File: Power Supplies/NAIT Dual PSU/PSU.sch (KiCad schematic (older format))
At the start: 41 parts, among them P1 120V, SW1 SW_Push_DPDT, SW2 SW_SPST_Lamp, T1 50V CT 100VA, U1 LM317_TO-220, U2 LM337_TO220

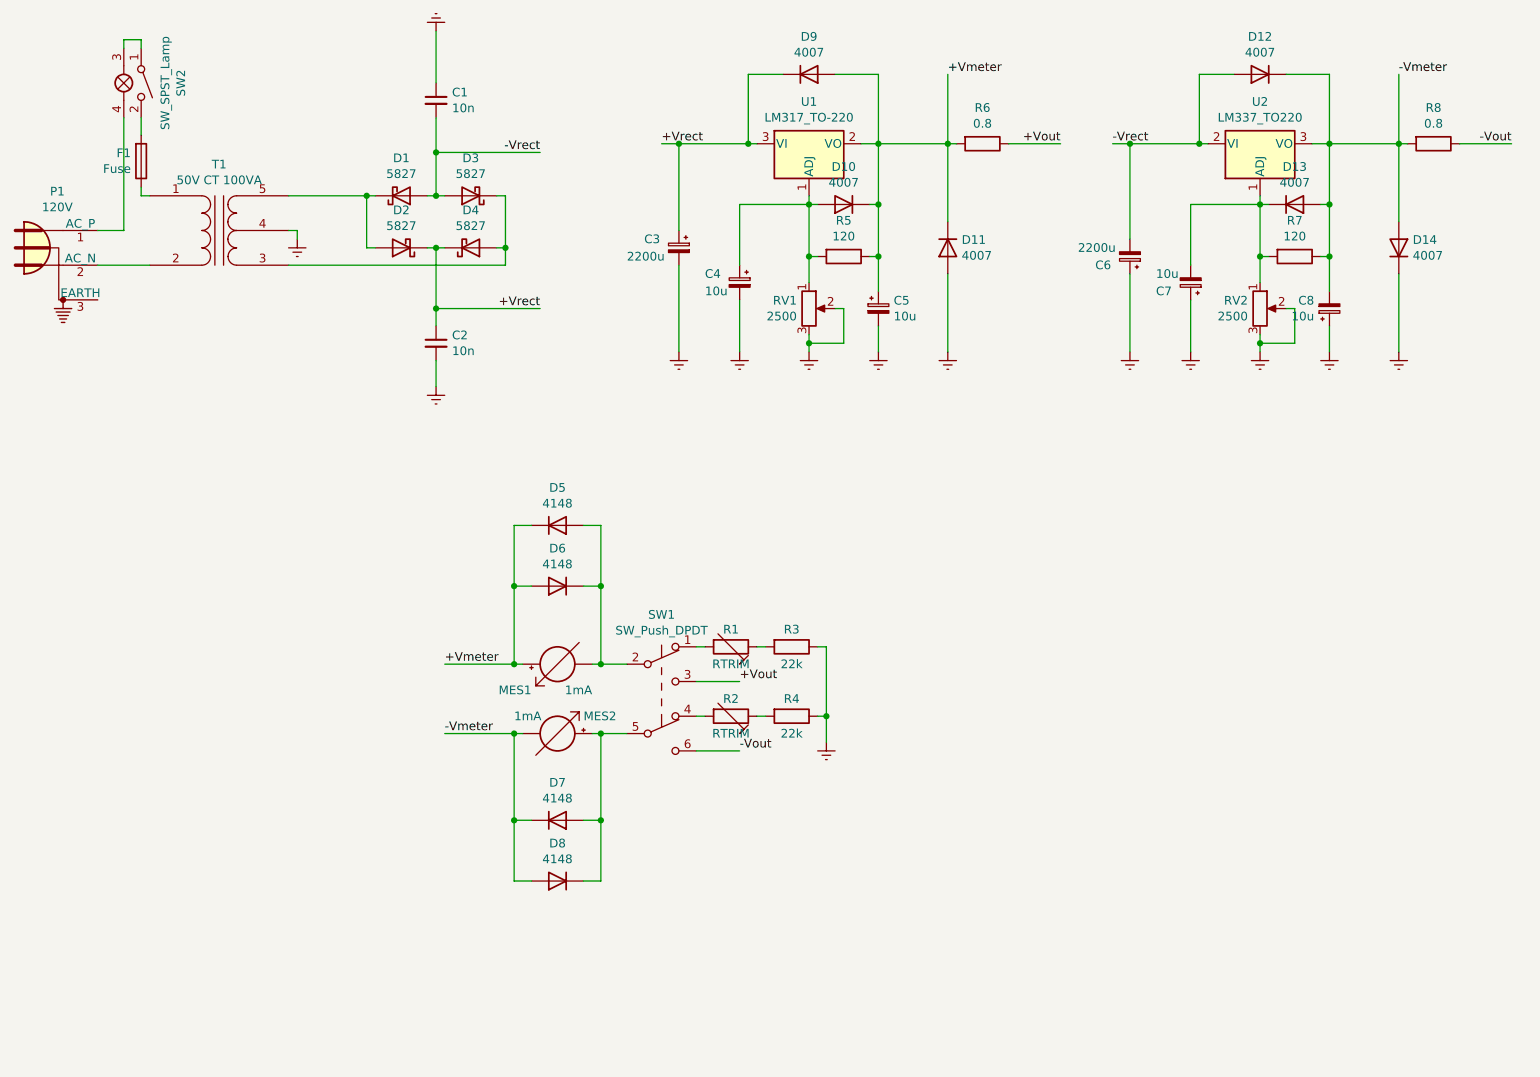
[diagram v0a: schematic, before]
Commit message: add new circuits
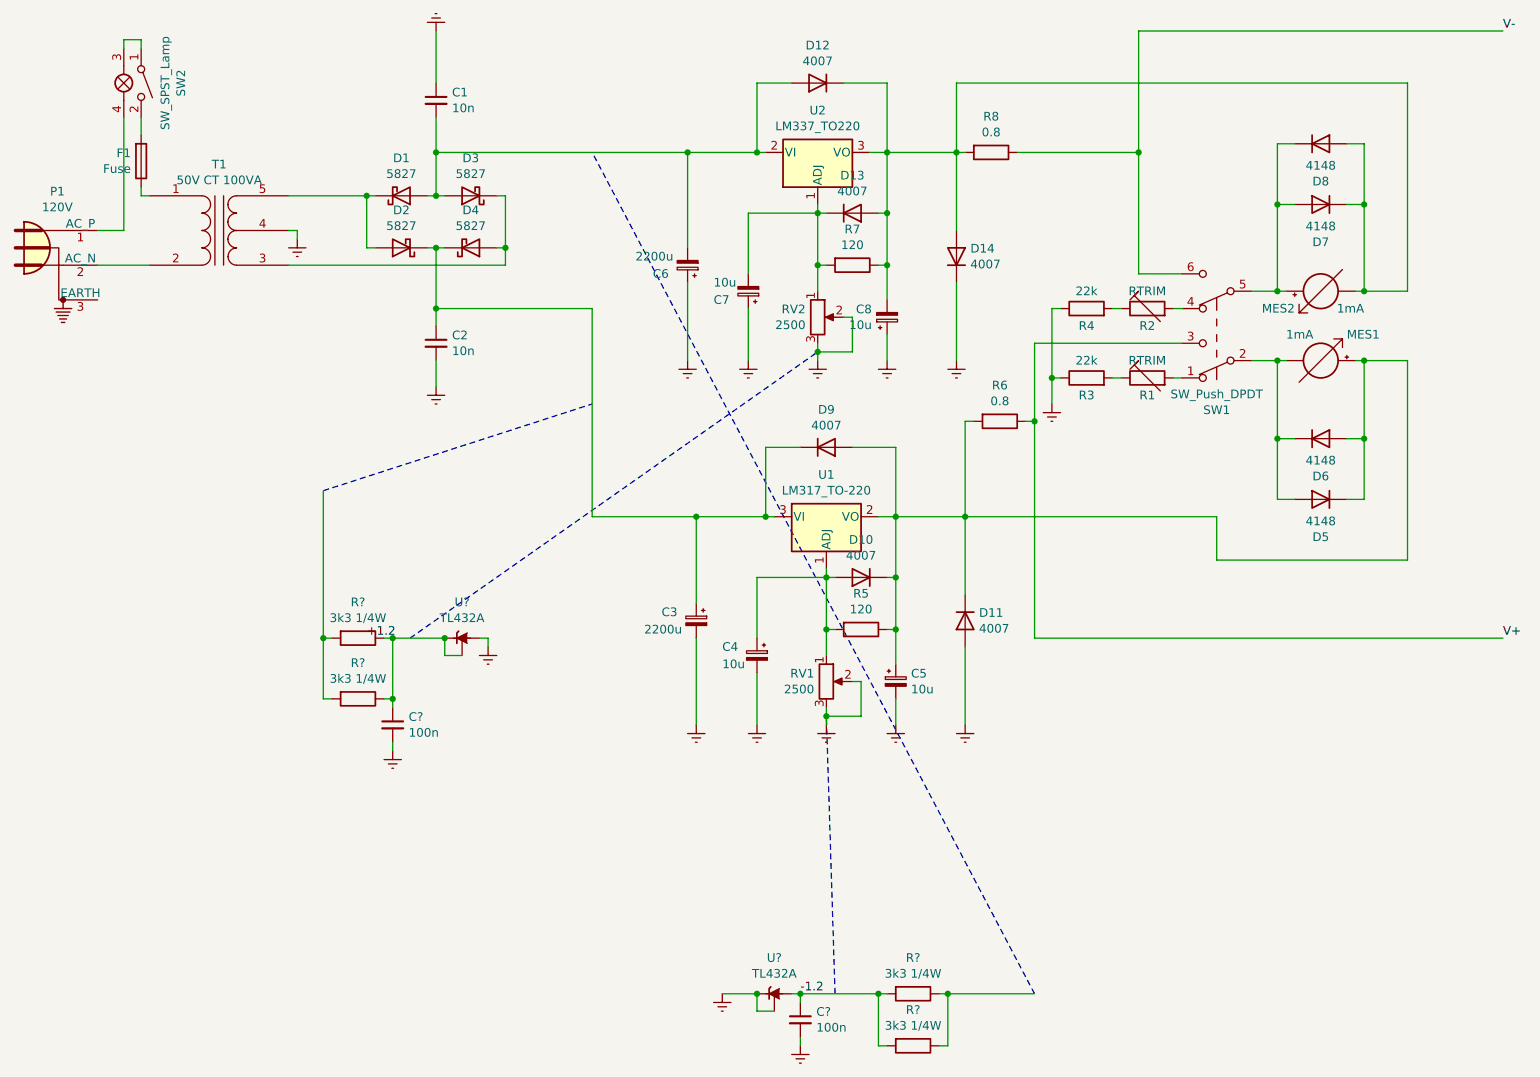
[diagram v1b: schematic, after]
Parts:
- added C? (x2): 100n, symbol Device:C_Small
- added R? (x4): 3k3 1/4W, symbol Device:R
- added U? (x2): TL432A, Package_TO_SOT_THT:TO-92_Inline, symbol Reference_Voltage:TL431LP
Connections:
- net Earth: now also C?.2, C?.2, U?.1 (REF), U?.2 (A), U?.3 (K)
- net +Vmeter: no longer names the net of C5.1, D10.1 (K), D11.1 (K), D5.1 (K), D6.2 (A), D9.2 (A), MES1.2 (+), R5.1, R6.2, U1.2 (VO)
- net +Vout renamed V+
- net +Vrect: no longer names the net of C2.1, C3.1, D2.1 (K), D4.1 (K), D9.1 (K), U1.3 (VI)
- net -Vmeter: no longer names the net of C8.2, D12.1 (K), D13.2 (A), D14.2 (A), D7.1 (K), D8.2 (A), MES2.1 (-), R7.1, R8.2, U2.3 (VO)
- net -Vout renamed V-
- net -Vrect: no longer names the net of C1.2, C6.2, D1.2 (A), D12.2 (A), D3.2 (A), U2.2 (VI)
- new net: C?.1, R?.1, R?.1, U?.1 (REF), U?.3 (K)
- new net: R?.2, R?.2
- new net: R?.1, R?.1
- new net -1.2: C?.1, R?.2, R?.2, U?.2 (A)
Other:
- moved on the sheet: C3, C4, C5, C6, C7, C8, D10, D11, D12, D13, D14, D5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
